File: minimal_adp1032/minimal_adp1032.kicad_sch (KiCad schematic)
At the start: 63 parts, among them J1 FW-02-03-G-D-085-155, J2 FW-02-03-G-D-085-155, J3 FW-07-03-G-D-085-155, J4 FW-07-03-G-D-085-155, J5 FW-02-03-G-D-085-155, J6 FW-02-03-G-D-085-155, T1 ZA9644-AED, U1 ADP1032ACPZ-5-R7

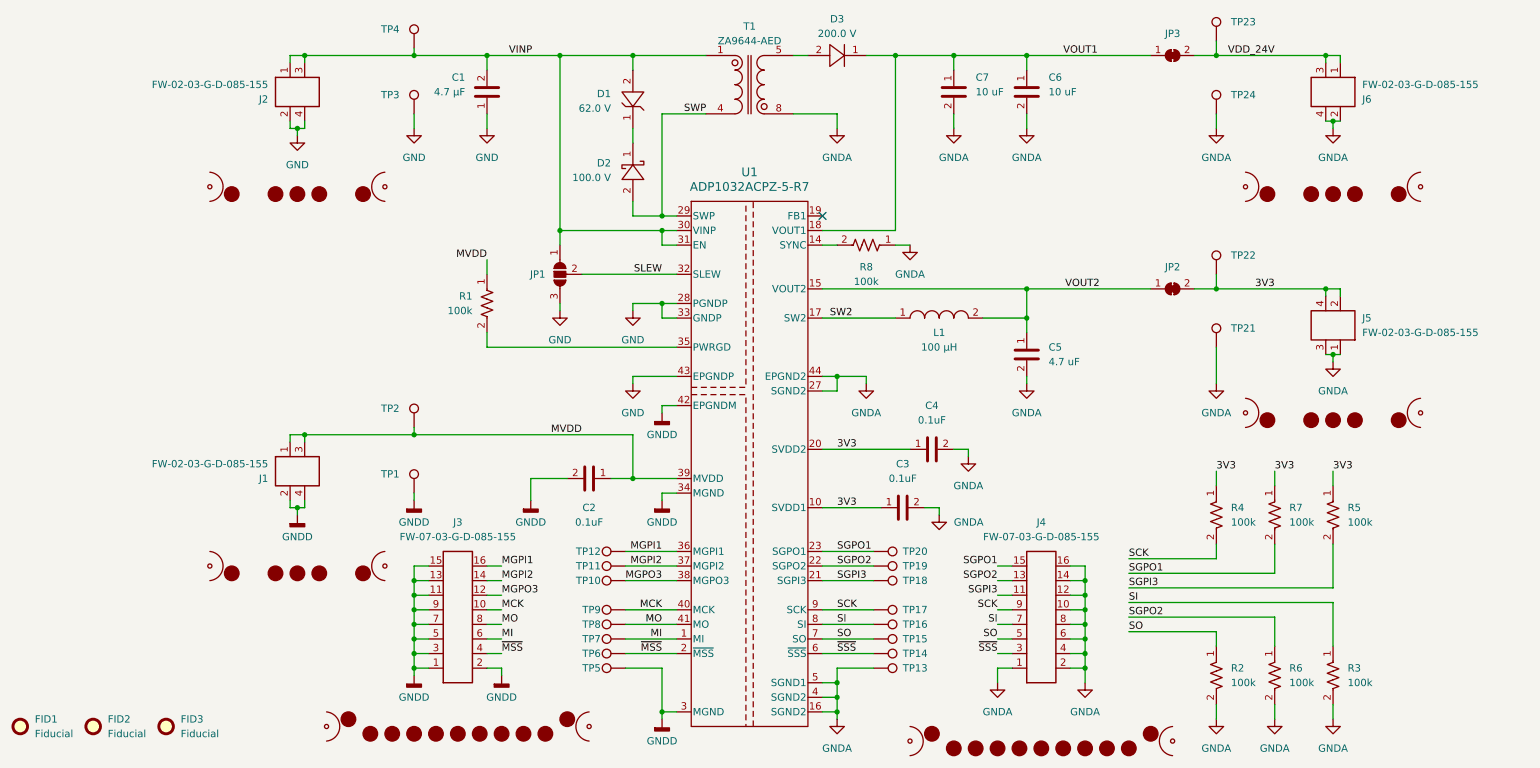
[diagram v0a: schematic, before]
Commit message: Switch to KiCad 9
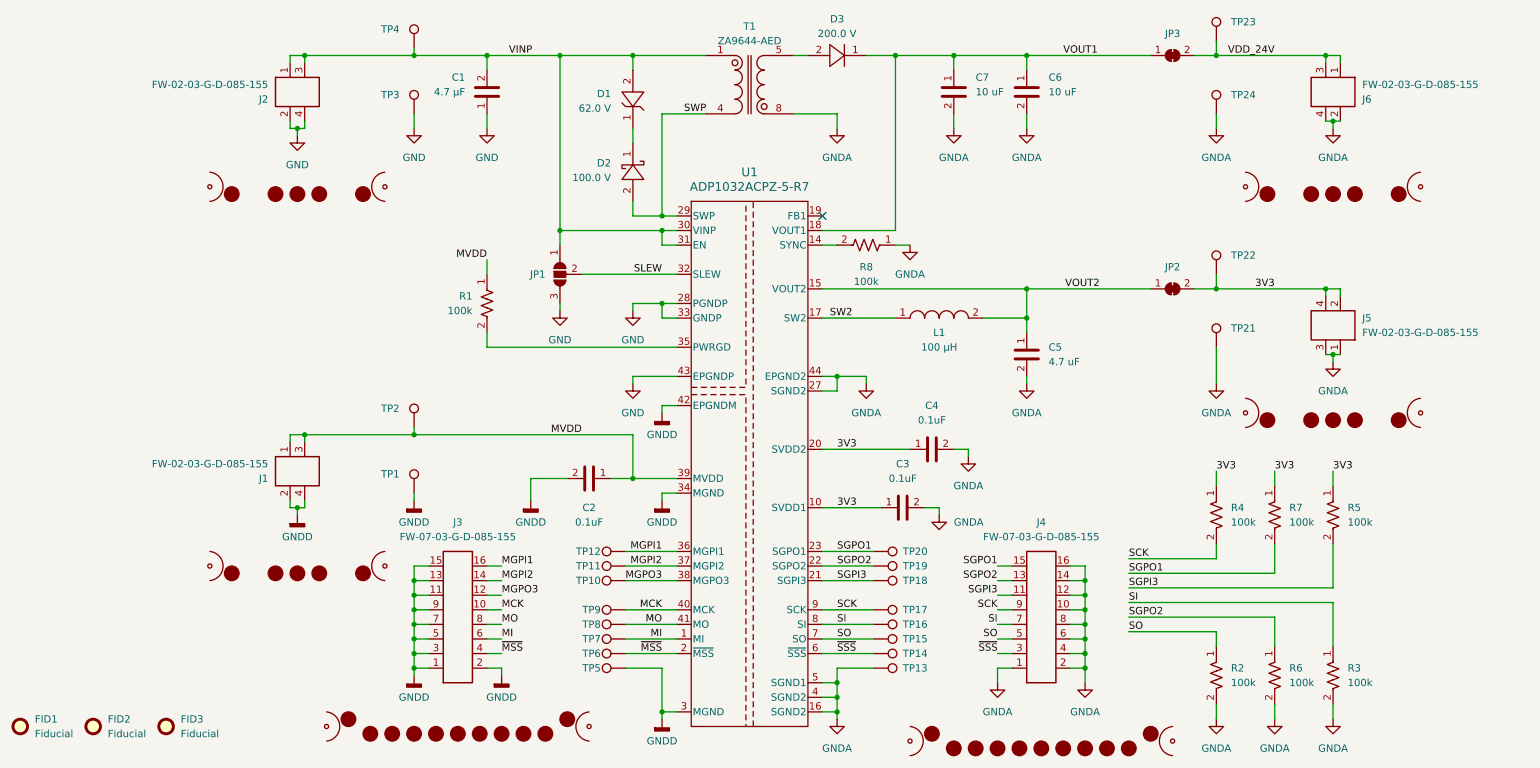
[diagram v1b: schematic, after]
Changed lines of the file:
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@@
 (kicad_sch
-	(version 20231120)
+	(version 20250114)
 	(generator "eeschema")
-	(generator_version "8.0")
+	(generator_version "9.0")
 	(paper "A3")
 	(junction
@@
 		)
 	)
+	(embedded_fonts no)
 )
